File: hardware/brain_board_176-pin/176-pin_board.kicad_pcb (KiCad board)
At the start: 4 copper layers, 61.8 x 73.2 mm, 77 parts, among them J1 MINI-USB-5P-3400020P1, P1 CONN_25X2, P10 CONN_2X2, P11 CONN_4X2, P12 CONN_4X2, P13 CONN_8X2, P2 CONN_25X2, P3 CONN_2, P4 CONN_6, P5 CONN_1, P6 CONN_2X2, P7 CONN_4X2, P8 CONN_4X2, P9 CONN_4X2, SW1 SW_PUSH, U1 STM32F407IGT6, U2 NUF2101MT1G, U3 LM2937, X1 CRYSTAL, X2 CRYSTAL(MC306)

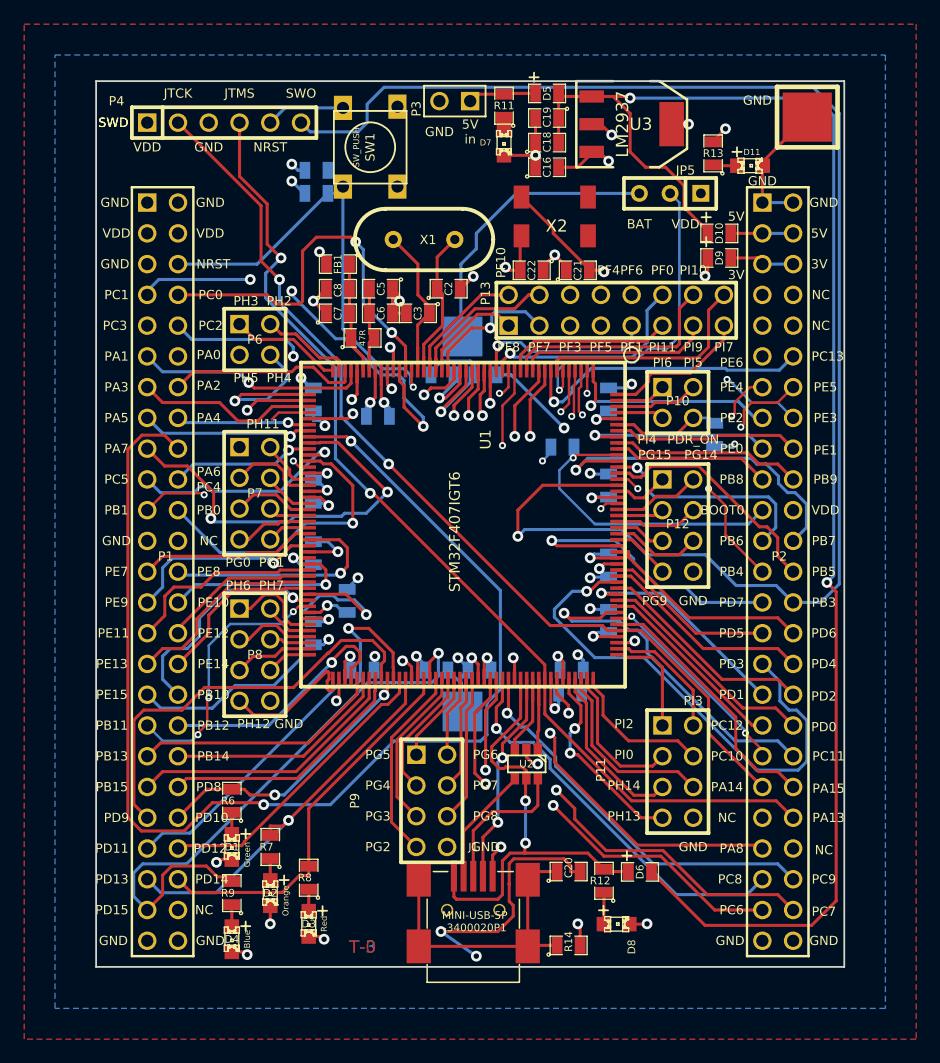
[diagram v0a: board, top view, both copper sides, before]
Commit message: update pcb files
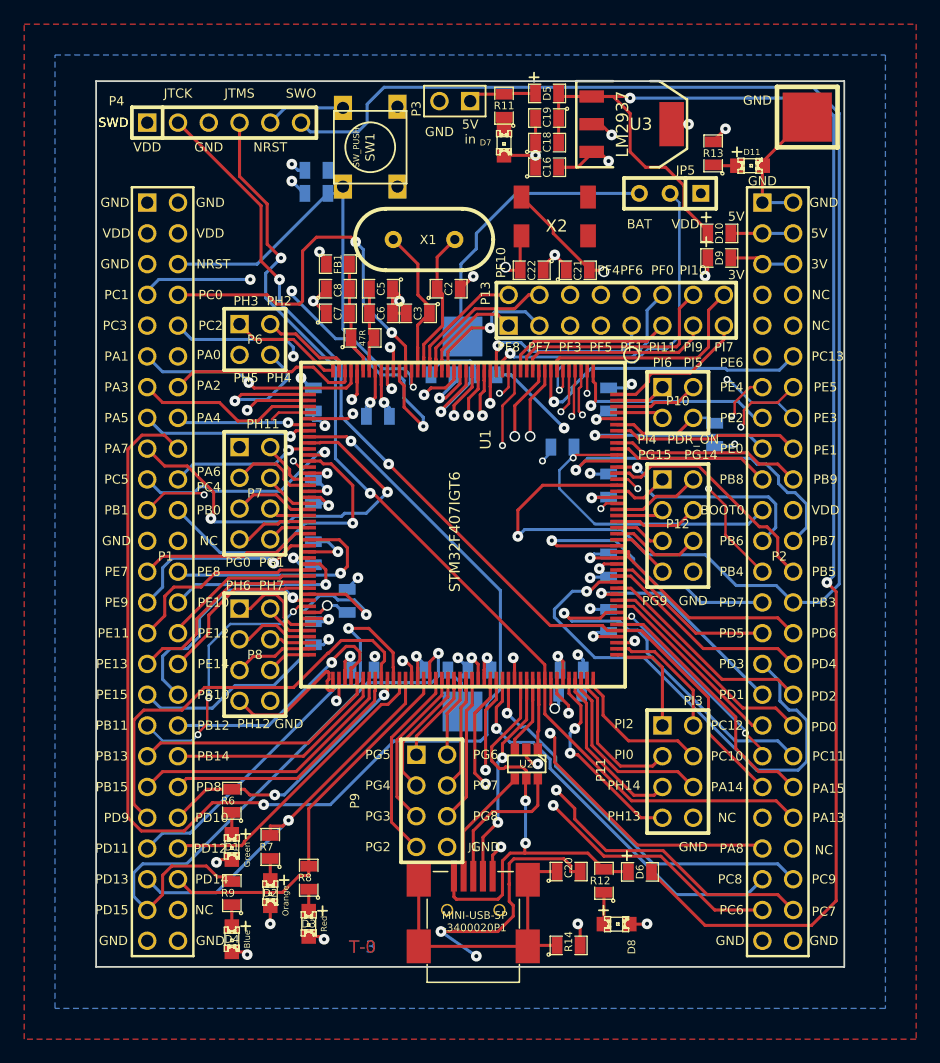
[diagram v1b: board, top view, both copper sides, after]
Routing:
- added copper zone on In2.Cu, net /VDD
- added copper zone on In1.Cu, net GND
- removed copper zone on PWR, net /VDD
- removed copper zone on GND, net GND
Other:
- net class Default removed
- net class smallest removed
